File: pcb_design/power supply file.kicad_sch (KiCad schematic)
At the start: 28 parts, among them Q1 AO3401A, Q2 AO3401A, U1 LT8610EMSE#PBF, U2 110k 0603, U3 L78M05CDT, U4 L78M05CDT

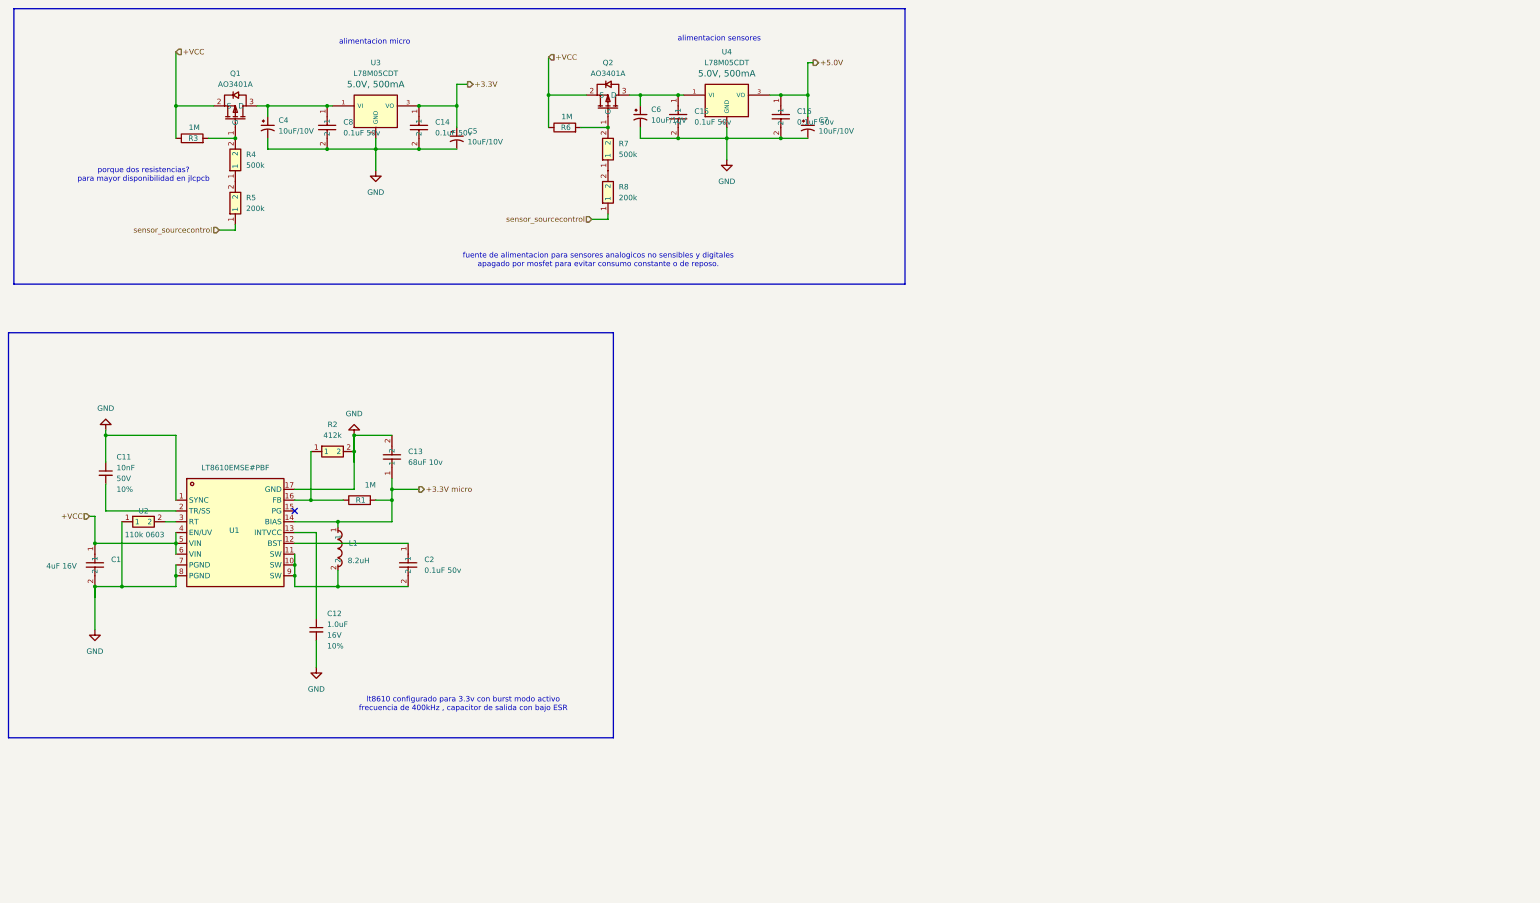
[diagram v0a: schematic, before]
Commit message: rediseno de esquematicos, rediseno de enrutado de pcb, eleccion de componentes basics
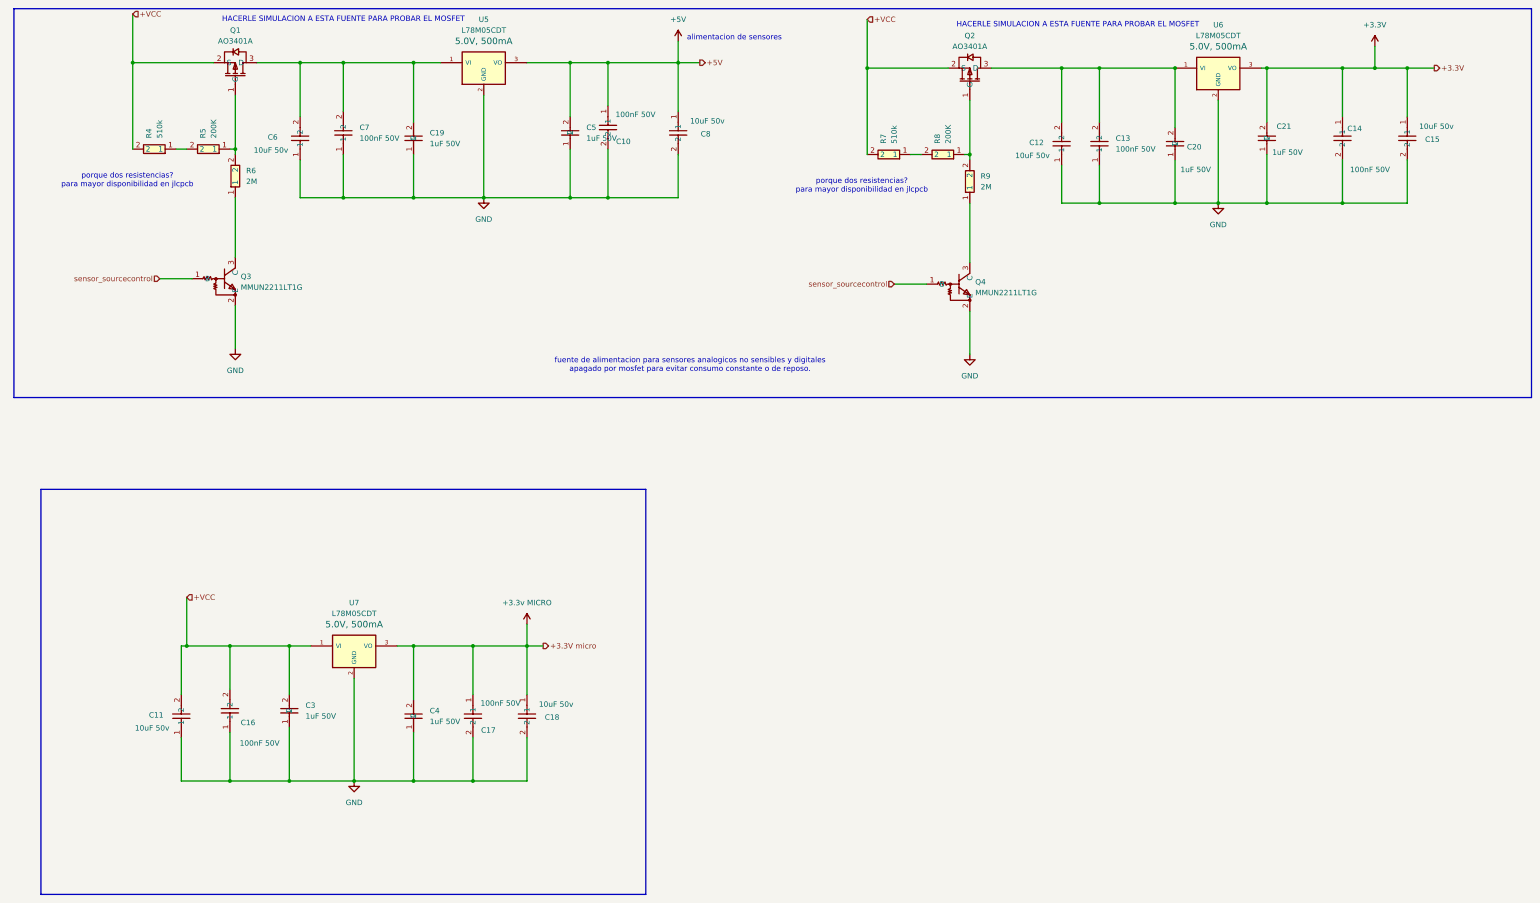
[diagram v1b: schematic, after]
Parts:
- removed C1: 4uF 16V, EasyEDA:C0603, symbol EasyEDA:CL10A475KO8NNNC
- removed C11: 10nF, PCM_SparkFun-Capacitor:C_0603_1608Metric, symbol PCM_SparkFun-Capacitor:10nF_0603_50V_10%
- removed C12: 1.0uF, PCM_SparkFun-Capacitor:C_0603_1608Metric, symbol PCM_SparkFun-Capacitor:1.0uF_0603_16V_10%
- removed C13: 68uF 10v, EasyEDA:C1206, symbol EasyEDA:C3216X5R1A686M160AC
- removed C14, C15, C16, C2, C8: 0.1uF 50v, EasyEDA:C0603, symbol EasyEDA:CL10B104KB8NNNC
- removed C4, C5, C6, C7: 10uF_4x5.3_10V, Capacitor_SMD:CP_Elec_4x5.3, symbol PCM_4ms_Capacitor:10uF_4x5.3_10V
- removed L1: 8.2uH, EasyEDA:IND-SMD_L7.0-W6.6_FXL0630, symbol EasyEDA:FXL0630-8R2-M
- removed R1, R3, R6: 1M_0603, PCM_4ms_Resistor:R_0603, symbol PCM_4ms_Resistor:1M_0603
- removed R2: 412k, EasyEDA:R1206, symbol EasyEDA:RT1206BRD07412KL
- removed R4, R7: 500k, EasyEDA:R0805, symbol EasyEDA:ARG05BTC5003
- removed R5, R8: 200k, EasyEDA:R0805, symbol EasyEDA:FRC0805F2003TS
- removed U1: LT8610EMSE#PBF, EasyEDA:MSOP-16_L4.0-W3.0-P0.50-LS4.9-BL-EP, symbol EasyEDA:LT8610EMSE#PBF
- removed U2: 110k 0603, EasyEDA:R0603, symbol EasyEDA:FRC0603F1103TS
- removed U3, U4: L78M05CDT, 4ms_Package_TO:TO-252-2, symbol PCM_4ms_Regulator:L78M05CDT
- added C10, C13, C14, C16, C17, C7: 100nF 50V, EasyEDA:C0603, symbol EasyEDA:CC0603KRX7R9BB104
- added C11, C12, C15, C18, C6, C8: 10uF 50v, EasyEDA:C0805, symbol EasyEDA:GRM21BR61H106KE43L
- added C19, C20, C21, C3, C4, C5: 1uF 50V, EasyEDA:C0805, symbol EasyEDA:CL21B105KBFNNNE
- added Q3, Q4: MMUN2211LT1G, EasyEDA:SOT-23-3_L2.9-W1.6-P1.90-LS2.8-BR, symbol EasyEDA:MMUN2211LT1G
- added R4, R7: 510k, EasyEDA:R0603, symbol EasyEDA:0603WAF5103T5E
- added R5, R8: 200K, EasyEDA:R0603, symbol EasyEDA:0603WAF2003T5E
- added R6, R9: 2M, EasyEDA:R0603, symbol EasyEDA:0603WAF2004T5E
- added U5, U6, U7: L78M05CDT, PCM_4ms_Package_TO:TO-220-3_Vertical, symbol PCM_4ms_Regulator:L78M05CDT
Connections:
- net +3.3V: now also C14.1, C15.1, C21.2, U6.3 (VO)
- net +VCC: now also C11.2, C16.2, C3.2, R4.2, R7.2, U7.1 (VI)
- net GND: now also C10.2, C11.1, C12.1, C13.1, C14.2, C15.2, C16.1, C17.2, C18.2, C19.1, C20.1, C21.1, C3.1, C4.1, C5.1, C6.1, C7.1, C8.2, Q3.2 (E), Q4.2 (E), U5.2 (GND), U6.2 (GND), U7.2 (GND)
- net sensor_sourcecontrol: now also Q3.1 (B), Q4.1 (B)
- net at Q2.1 (G): now also R8.1, R9.2
- net at Q1.1 (G): now also R5.1, R6.2
- net at Q2.3 (D): now also C12.2, C13.2, C20.2, U6.1 (VI)
- net at Q1.3 (D): now also C19.2, C6.2, C7.2, U5.1 (VI)
- new net: R4.1, R5.2
- new net: Q4.3 (C), R9.1
- new net: Q3.3 (C), R6.1
- new net: R7.1, R8.2
- new net +3.3v MICRO: C17.1, C18.1, C4.2, U7.3 (VO)
- new net +5V: C10.1, C5.2, C8.1, U5.3 (VO)
- no-connect marks 1 -> 0
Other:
- note added: "HACERLE SIMULACION A ESTA FUENTE PARA PROBAR EL MOSFET"
- note added: "alimentacion de sensores"
- note removed: "alimentacion micro"
- note removed: "alimentacion sensores"
- note removed: "lt8610 configurado para 3.3v con burst modo activo frecuencia de 400kHz , capacitor de salida con bajo ESR"
- moved on the sheet: Q1
